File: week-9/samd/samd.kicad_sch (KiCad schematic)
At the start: 17 parts, among them J1 PinSocket_01x05_P2.54mm_Verti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, J2 PinSocket_01x05_P2.54mm_Verti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, J3 PinSocket_01x05_P2.54mm_Verti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, J4 PinSocket_01x05_P2.54mm_Verti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, J5 PinSocket_01x03_P2.54mm_Verti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, J6 PinSocket_01x03_P2.54mm_Verti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, P1 Conn_USB_A_Socket_AdamTech_US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, U1 ATSAMD21E17A-A, U3 AMS1117

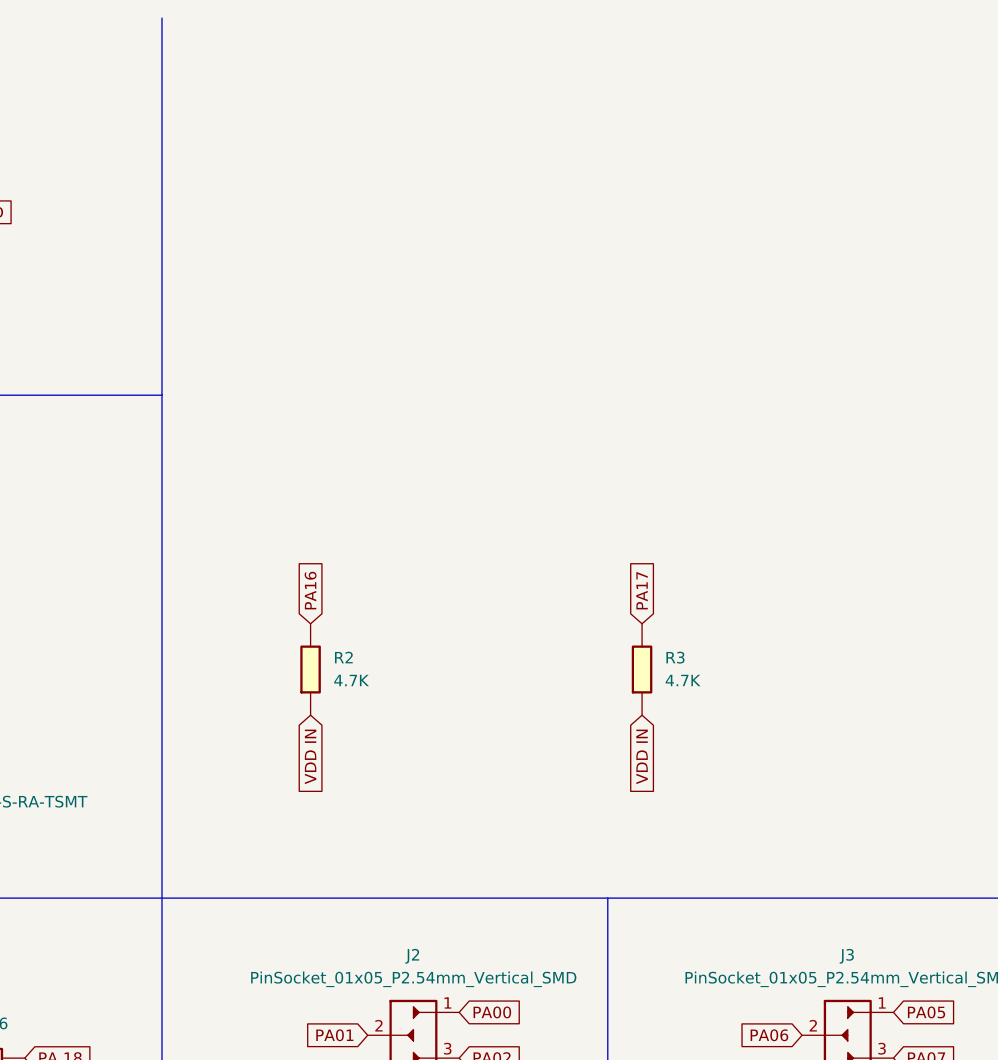
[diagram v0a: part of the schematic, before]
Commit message: week-9
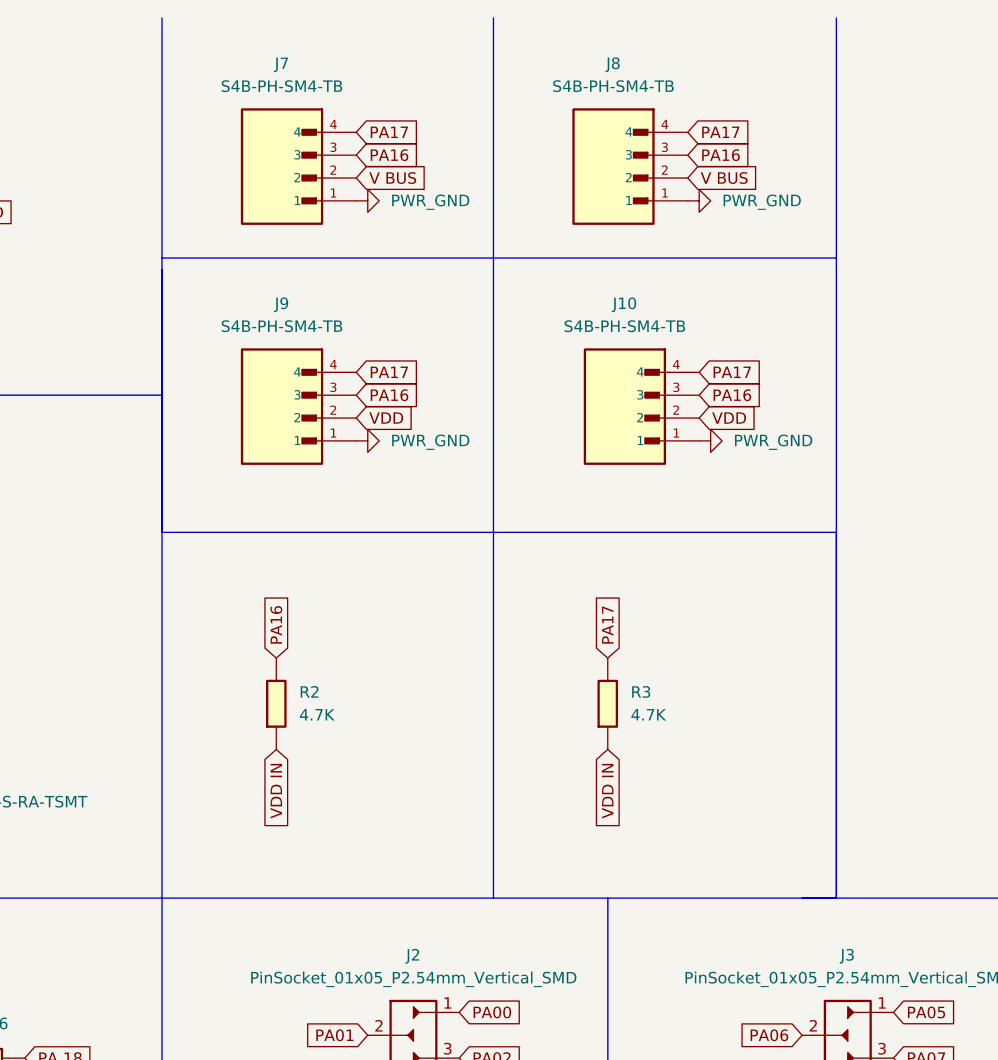
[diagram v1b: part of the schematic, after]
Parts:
- added J10, J7, J8, J9: S4B-PH-SM4-TB, S4B-PH-SM4-TB:JST_S4B-PH-SM4-TB, symbol S4B-PH-SM4-TB:S4B-PH-SM4-TB
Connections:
- net PA16: now also J10.3, J7.3, J8.3, J9.3
- net PA17: now also J10.4, J7.4, J8.4, J9.4
- net PWR_GND: now also J10.1, J7.1, J8.1, J9.1
- net V BUS: now also J7.2, J8.2
- net VDD: now also J10.2, J9.2
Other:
- moved on the sheet: R2, R3
